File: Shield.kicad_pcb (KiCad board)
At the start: 2 copper layers, 54.6 x 53.6 mm, 33 parts, among them J1 Screw_Terminal_01x03, J2 Screw_Terminal_01x03, J3 Screw_Terminal_01x03, J4 Screw_Terminal_01x03, U1 SPX3819M5-L-3-3, U2 SPX3819M5-L-3-3, U3 MAX31865xTP, U4 MAX31865xTP, U5 MAX31865xTP, U6 MAX31865xTP

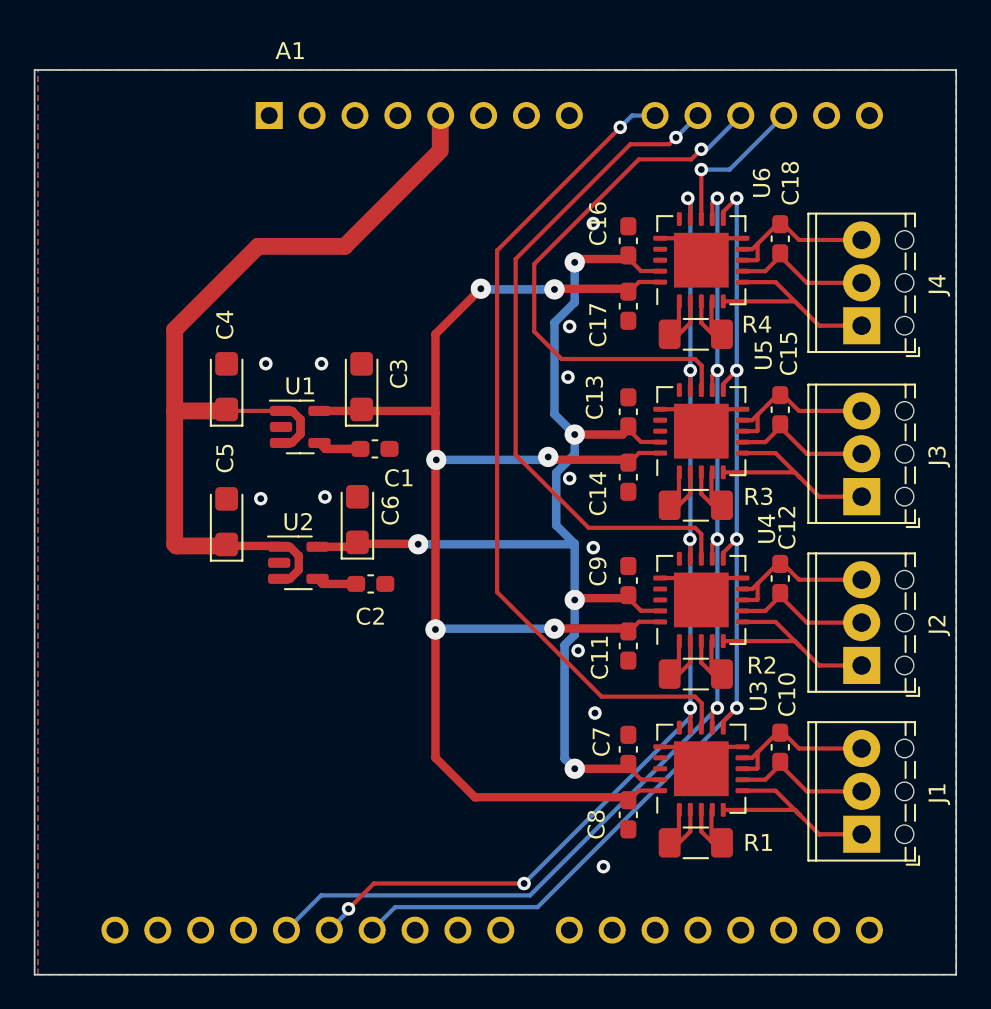
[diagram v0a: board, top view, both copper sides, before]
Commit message: v002
AJoute des grains de café pour choisir le chip select
Miroir connecteur arduiono
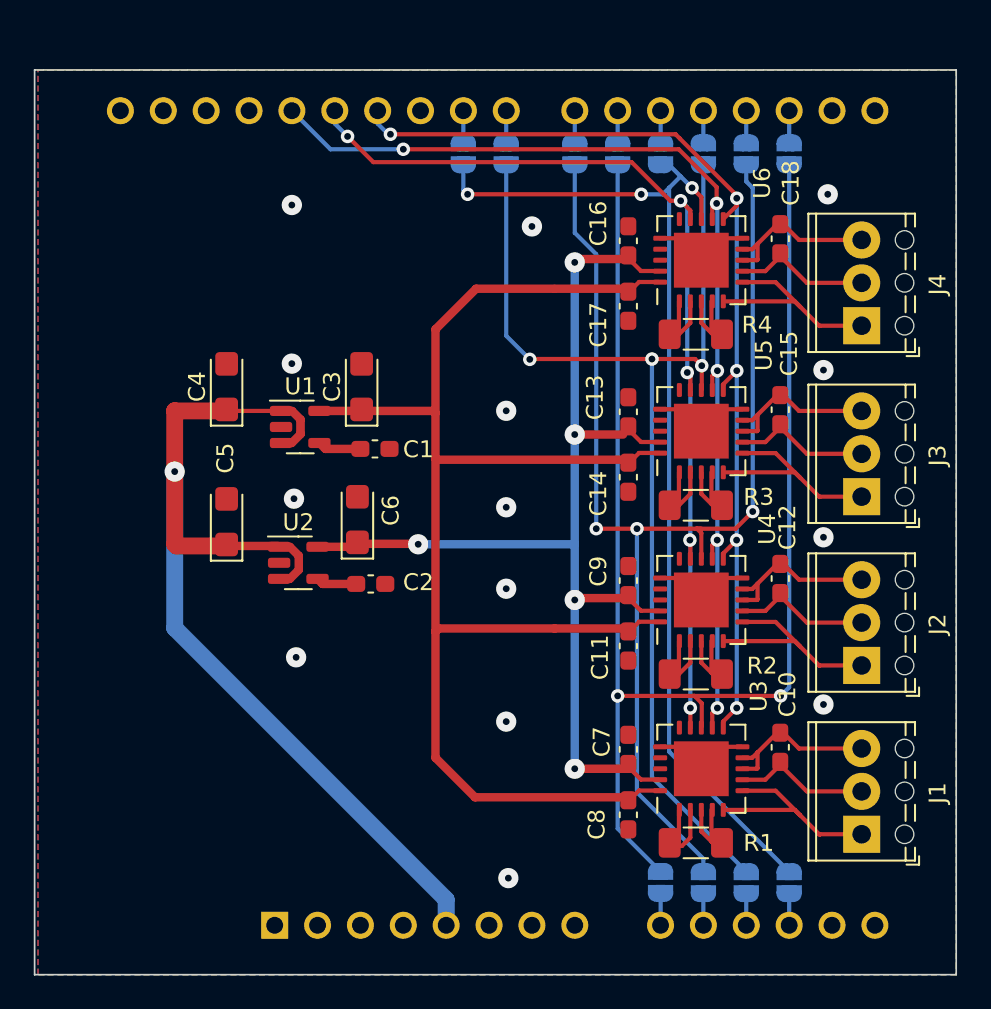
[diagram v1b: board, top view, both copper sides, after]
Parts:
- added JP1: SolderJumper_2_Open, Jumper:SolderJumper-2_P1.3mm_Open_RoundedPad1.0x1.5mm, B.Cu at (144.7, 44.8)
- added JP10: SolderJumper_2_Bridged, Jumper:SolderJumper-2_P1.3mm_Open_RoundedPad1.0x1.5mm, B.Cu at (139.6, 87.9)
- added JP11: SolderJumper_2_Bridged, Jumper:SolderJumper-2_P1.3mm_Open_RoundedPad1.0x1.5mm, B.Cu at (142.2, 87.9)
- added JP12: SolderJumper_2_Bridged, Jumper:SolderJumper-2_P1.3mm_Open_RoundedPad1.0x1.5mm, B.Cu at (144.7, 87.9)
- added JP2: SolderJumper_2_Open, Jumper:SolderJumper-2_P1.3mm_Open_RoundedPad1.0x1.5mm, B.Cu at (142.2, 44.8)
- added JP3: SolderJumper_2_Open, Jumper:SolderJumper-2_P1.3mm_Open_RoundedPad1.0x1.5mm, B.Cu at (139.6, 44.8)
- added JP4: SolderJumper_2_Open, Jumper:SolderJumper-2_P1.3mm_Open_RoundedPad1.0x1.5mm, B.Cu at (137.1, 44.8)
- added JP5: SolderJumper_2_Open, Jumper:SolderJumper-2_P1.3mm_Open_RoundedPad1.0x1.5mm, B.Cu at (134.5, 44.8)
- added JP6: SolderJumper_2_Open, Jumper:SolderJumper-2_P1.3mm_Open_RoundedPad1.0x1.5mm, B.Cu at (132.0, 44.8)
- added JP7: SolderJumper_2_Open, Jumper:SolderJumper-2_P1.3mm_Open_RoundedPad1.0x1.5mm, B.Cu at (127.9, 44.8)
- added JP8: SolderJumper_2_Open, Jumper:SolderJumper-2_P1.3mm_Open_RoundedPad1.0x1.5mm, B.Cu at (125.4, 44.8)
- added JP9: SolderJumper_2_Bridged, Jumper:SolderJumper-2_P1.3mm_Open_RoundedPad1.0x1.5mm, B.Cu at (137.1, 87.9)
- A1: moved to B.Cu
- C1, C2: value 100 nf -> 100 nF
- C3, C6: value 10uf -> 10uF
- C4, C5: value 1uf -> 1uF
- moved A1 48.0 mm to (114.2, 90.5)
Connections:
- A1 pad 10: /CS_MAX2 -> Net-(A1-Pad10)
- A1 pad 11: /CS_MAX3 -> Net-(A1-Pad11)
- A1 pad 12: /CS_MAX4 -> Net-(A1-Pad12)
- A1 pad 17: unconnected-(A1-Pad17) -> Net-(A1-Pad17)
- A1 pad 18: unconnected-(A1-Pad18) -> Net-(A1-Pad18)
- A1 pad 19: unconnected-(A1-Pad19) -> Net-(A1-Pad19)
- A1 pad 20: unconnected-(A1-Pad20) -> Net-(A1-Pad20)
- A1 pad 21: unconnected-(A1-Pad21) -> Net-(A1-Pad21)
- A1 pad 22: unconnected-(A1-Pad22) -> Net-(A1-Pad22)
- A1 pad 23: unconnected-(A1-Pad23) -> Net-(A1-Pad23)
- A1 pad 24: unconnected-(A1-Pad24) -> Net-(A1-Pad24)
- A1 pad 9: /CS_MAX1 -> Net-(A1-Pad9)
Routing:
- net /CS_MAX4: track 9.14 -> 62.9 mm, vias 1 -> 3
- net /CS_MAX1: track 49.2 -> 86.4 mm, vias 1 -> 2
- net /CS_MAX3: track 32.1 -> 68.5 mm, vias 1 -> 3
- net /CS_MAX2: track 40.3 -> 76.6 mm, vias 1 -> 3
- net +5V: track 61.2 -> 67.7 mm, vias 0 -> 1
- net /SPI2_MISO: track 62.3 -> 58.2 mm, vias 6 -> 5
- net /SPI2_SCK: track 66.4 -> 62.7 mm, vias 4 -> 5
- net /SPI2_MOSI: track 63.3 -> 60.1 mm, vias 4 -> 5
- net +3.3V: track 68.5 -> 66.1 mm
- net Net-(A1-Pad23): track 0.00 -> 1.91 mm
- net Net-(A1-Pad24): track 0.00 -> 1.91 mm
- net Net-(A1-Pad22): track 0.00 -> 1.91 mm
- net Net-(A1-Pad21): track 0.00 -> 1.91 mm
- net Net-(A1-Pad20): track 0.00 -> 1.91 mm
- net Net-(A1-Pad19): track 0.00 -> 1.91 mm
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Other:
- board text added: "CS1 : JP1 or JP5 or JP9 CS1 : JP2 or JP6 or JP10 CS1 : JP3 or JP7 or JP11 CS1 : JP4 or JP8 or JP12 PCB v002 Mula Gabriel"
